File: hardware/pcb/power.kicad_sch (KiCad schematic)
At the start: 4 parts, among them IC1 MCP16502, U3 MAX17260, U4 BQ25640

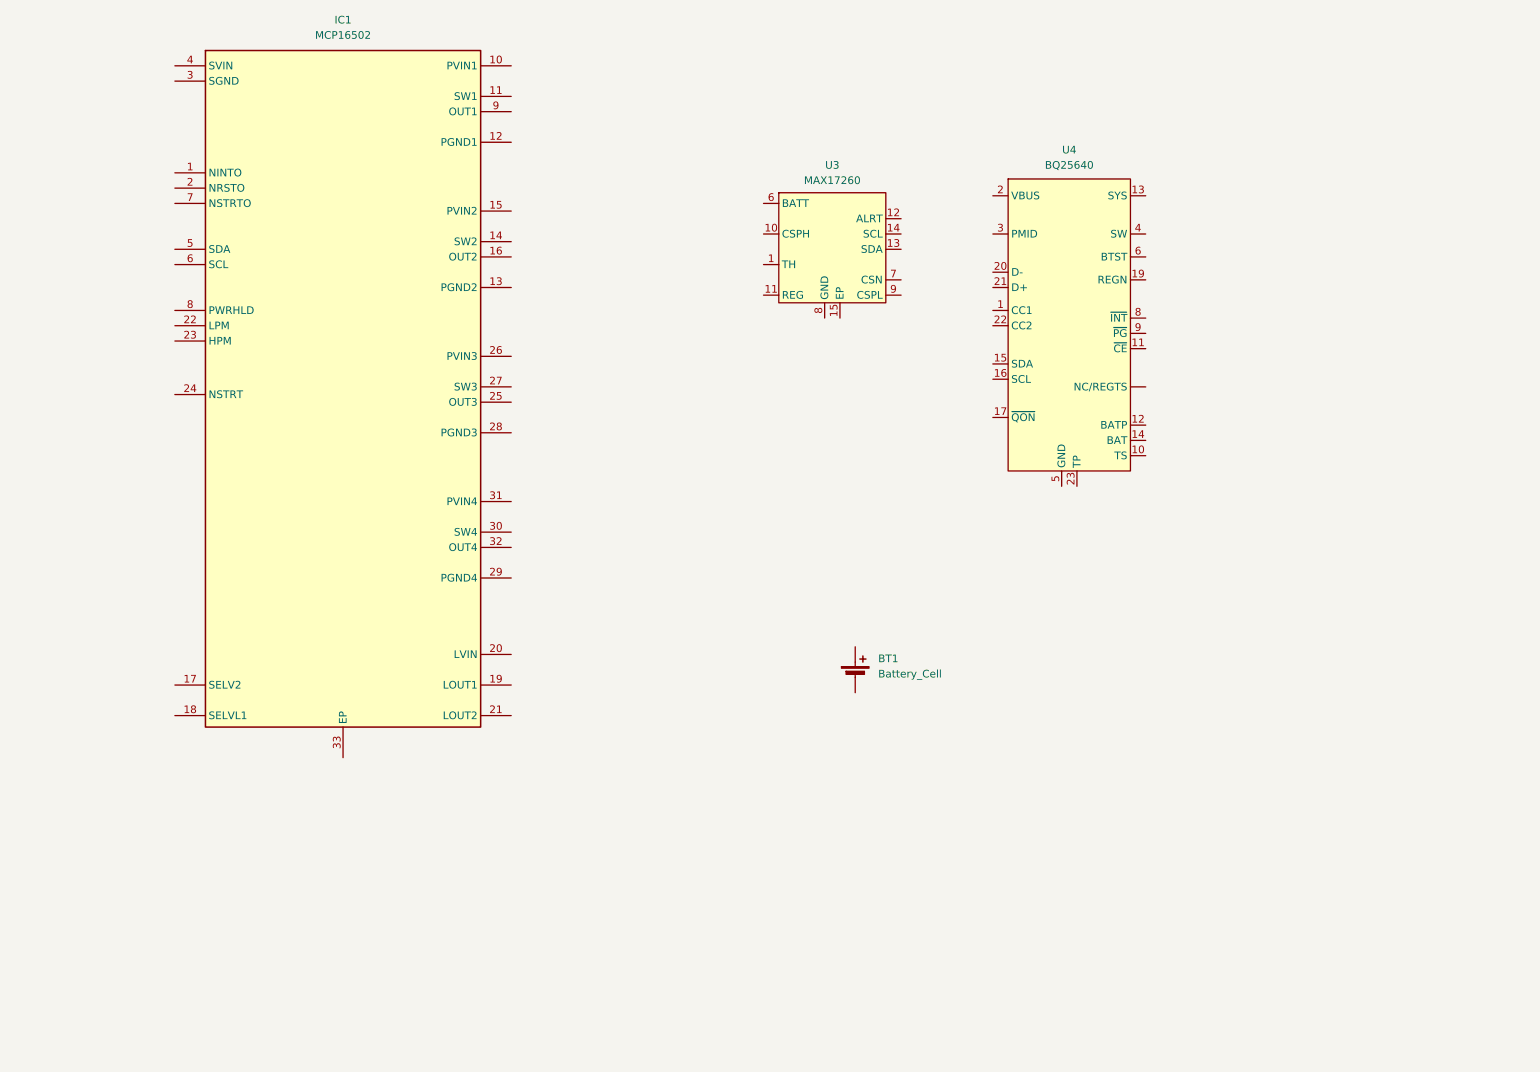
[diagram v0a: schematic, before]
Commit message: usb power
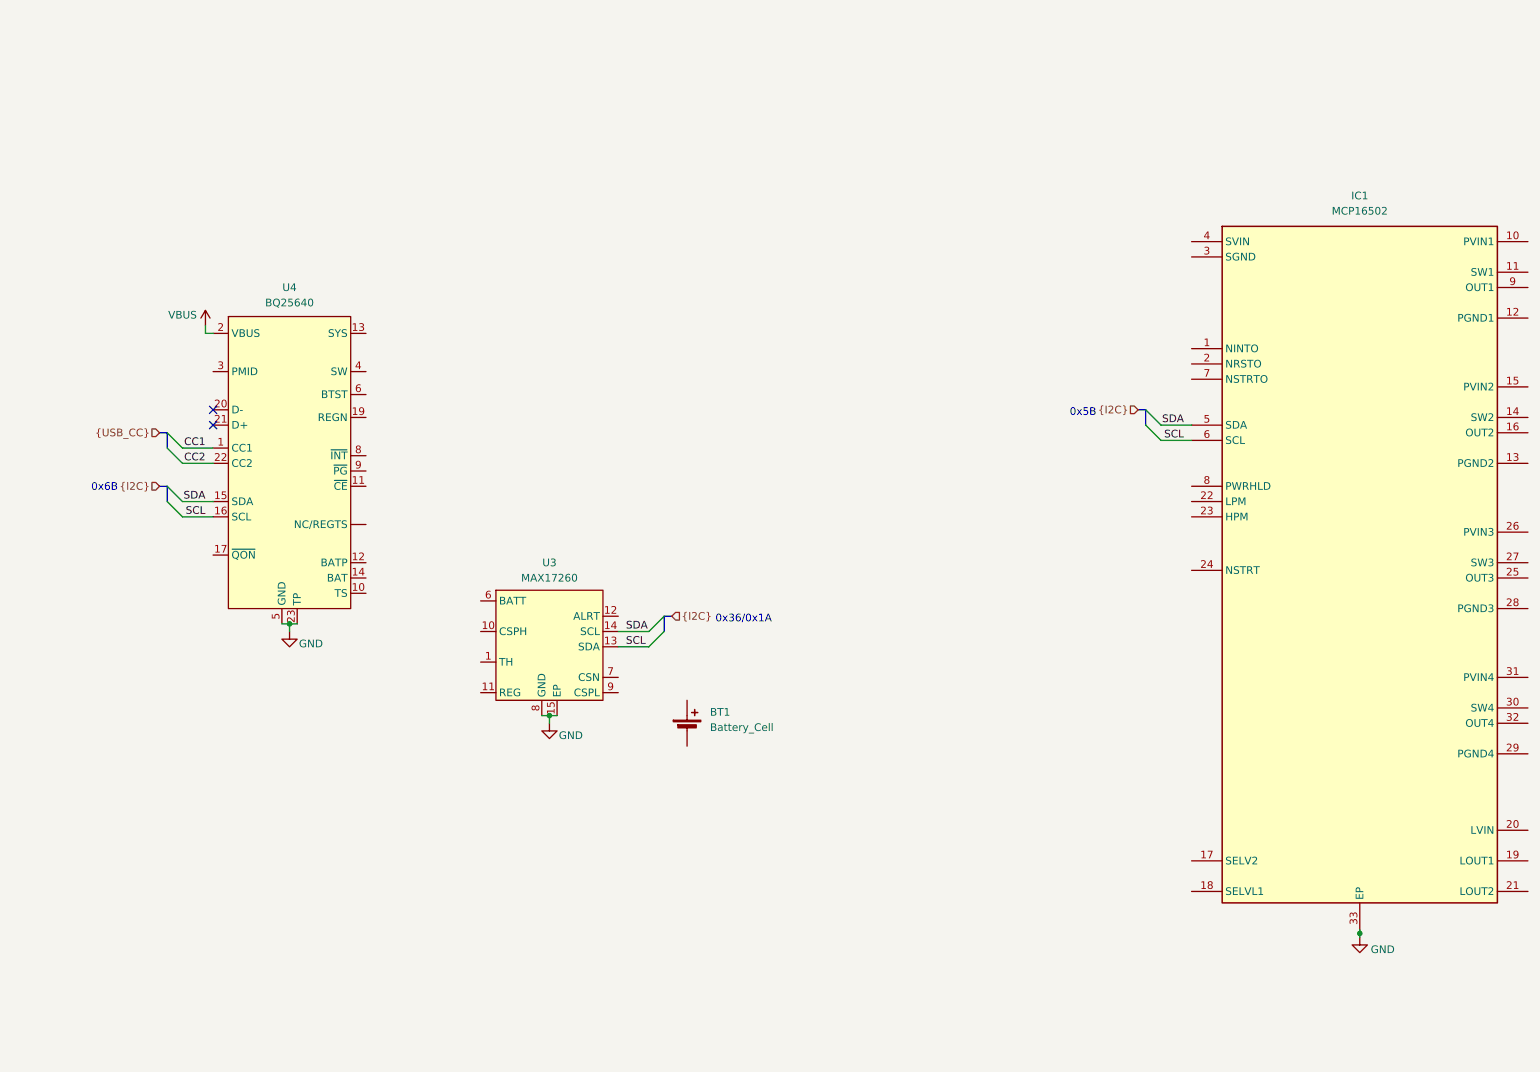
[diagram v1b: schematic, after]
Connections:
- net GND: now also IC1.33 (EP), U3.15 (EP), U3.8 (GND), U4.23 (TP)
- net CC1: now reaches U4.1 (CC1)
- net SDA: now reaches U4.15 (SDA)
- net SDA: now also IC1.5 (SDA), U3.14 (SCL)
- net SCL: now reaches U4.16 (SCL)
- net SCL: now also IC1.6 (SCL), U3.13 (SDA)
- net VBUS: now reaches U4.2 (VBUS)
- net CC2: now reaches U4.22 (CC2)
- no-connect marks 0 -> 2
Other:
- note added: "0x36/0x1A"
- note added: "0x5B"
- note added: "0x6B"
- moved on the sheet: BT1, IC1, U3, U4

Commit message: finished power
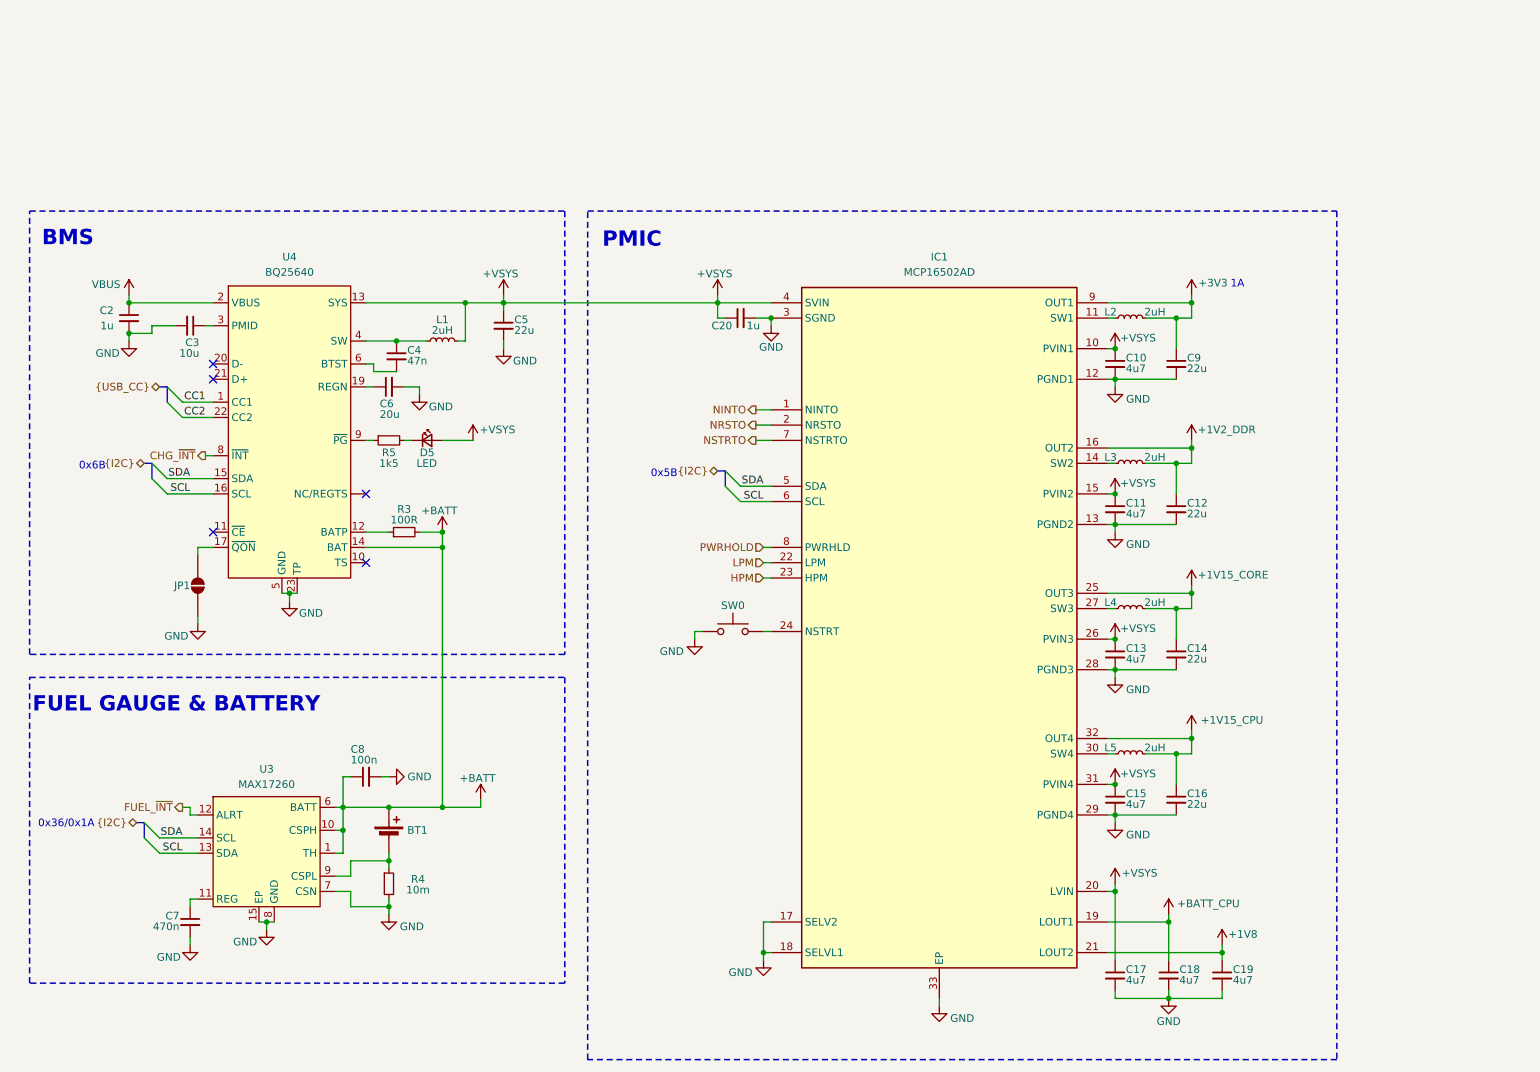
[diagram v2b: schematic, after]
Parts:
- added C10, C11, C13, C15, C17, C18, C19: 4u7, symbol Device:C_Small
- added C12, C14, C16, C5, C9: 22u, symbol Device:C_Small
- added C2, C20: 1u, symbol Device:C_Small
- added C3: 10u, symbol Device:C_Small
- added C4: 47n, symbol Device:C_Small
- added C6: 20u, symbol Device:C_Small
- added C7: 470n, symbol Device:C_Small
- added C8: 100n, symbol Device:C_Small
- added D5: LED, LED_SMD:LED_0603_1608Metric, symbol Device:LED_Small
- added JP1: SolderJumper_2_Open, symbol Jumper:SolderJumper_2_Open
- added L1, L2, L3, L4, L5: 2uH, symbol Device:L_Small
- added R3: 100R, symbol Device:R_Small
- added R4: 10m, symbol Device:R_Small
- added R5: 1k5, symbol Device:R_Small
- added SW0: SW_Push, symbol Switch:SW_Push
- IC1: value MCP16502 -> MCP16502AD
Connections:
- net GND: now also IC1.12 (PGND1), IC1.13 (PGND2), IC1.17 (SELV2), IC1.18 (SELVL1), IC1.28 (PGND3), IC1.29 (PGND4), IC1.3 (SGND), U3.7 (CSN), C10.2, C11.2, C12.2, C13.2, C14.2, C15.2, C16.2, C17.2, C18.2, C19.2, C2.2, C20.2, C3.2, C5.2, C6.2, C7.2, C8.2, C9.2, JP1.1 (A), R4.2, SW0.1
- net VBUS: now also C2.1
- net at U4.12 (BATP): now also R3.1
- net +VSYS: now reaches U4.13 (SYS)
- net +VSYS: now also IC1.10 (PVIN1), IC1.15 (PVIN2), IC1.20 (LVIN), IC1.26 (PVIN3), IC1.31 (PVIN4), IC1.4 (SVIN), C10.1, C11.1, C13.1, C15.1, C17.1, C20.1, C5.1, D5.2 (A), L1.2
- net +BATT: now reaches U4.14 (BAT)
- net +BATT: now also BT1.1 (+), U3.1 (TH), U3.10 (CSPH), U3.6 (BATT), C8.1, R3.2
- net at U4.17 (~{QON}): now also JP1.2 (B)
- net at U4.19 (REGN): now also C6.1
- net at U4.3 (PMID): now also C3.1
- net at U4.4 (SW): now also C4.1, L1.1
- net at U4.6 (BTST): now also C4.2
- net CHG_~{INT}: now reaches U4.8 (~{INT})
- net at U4.9 (~{PG}): now also R5.1
- net NINTO: now reaches IC1.1 (NINTO)
- net at IC1.11 (SW1): now also L2.1
- net at IC1.14 (SW2): now also L3.1
- net +1V2_DDR: now reaches IC1.16 (OUT2)
- net +1V2_DDR: now also C12.1, L3.2
- net +BATT_CPU: now reaches IC1.19 (LOUT1)
- net +BATT_CPU: now also C18.1
- net NRSTO: now reaches IC1.2 (NRSTO)
- net +1V8: now reaches IC1.21 (LOUT2)
- net +1V8: now also C19.1
- net LPM: now reaches IC1.22 (LPM)
- net HPM: now reaches IC1.23 (HPM)
- net at IC1.24 (NSTRT): now also SW0.2
- net +1V15_CORE: now reaches IC1.25 (OUT3)
- net +1V15_CORE: now also C14.1, L4.2
- net at IC1.27 (SW3): now also L4.1
- net at IC1.30 (SW4): now also L5.1
- net +1V15_CPU: now reaches IC1.32 (OUT4)
- net +1V15_CPU: now also C16.1, L5.2
- net NSTRTO: now reaches IC1.7 (NSTRTO)
- net PWRHOLD: now reaches IC1.8 (PWRHLD)
- net +3V3: now reaches IC1.9 (OUT1)
- net +3V3: now also C9.1, L2.2
- net at BT1.2 (-): now also U3.9 (CSPL), R4.1
- net at U3.11 (REG): now also C7.1
- net FUEL_~{INT}: now reaches U3.12 (ALRT)
- new net: D5.1 (K), R5.2
- no-connect marks 2 -> 5
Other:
- note added: "1A"
- note added: "BMS"
- note added: "FUEL GAUGE & BATTERY"
- note added: "PMIC"
- moved on the sheet: BT1, IC1, U3, U4
